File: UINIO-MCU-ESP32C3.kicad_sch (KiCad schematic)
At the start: 40 parts, among them J1 Conn_01x15_Male, J2 外接串行下载接口, J3 Conn_01x15_Male, SW1 复位按键, SW2 下载按键, U1 ME6211C33M5G-N, U2 W25Q128JVSSIQ, U3 ESP32-C3, U4 CH343P, Y1 40MHz

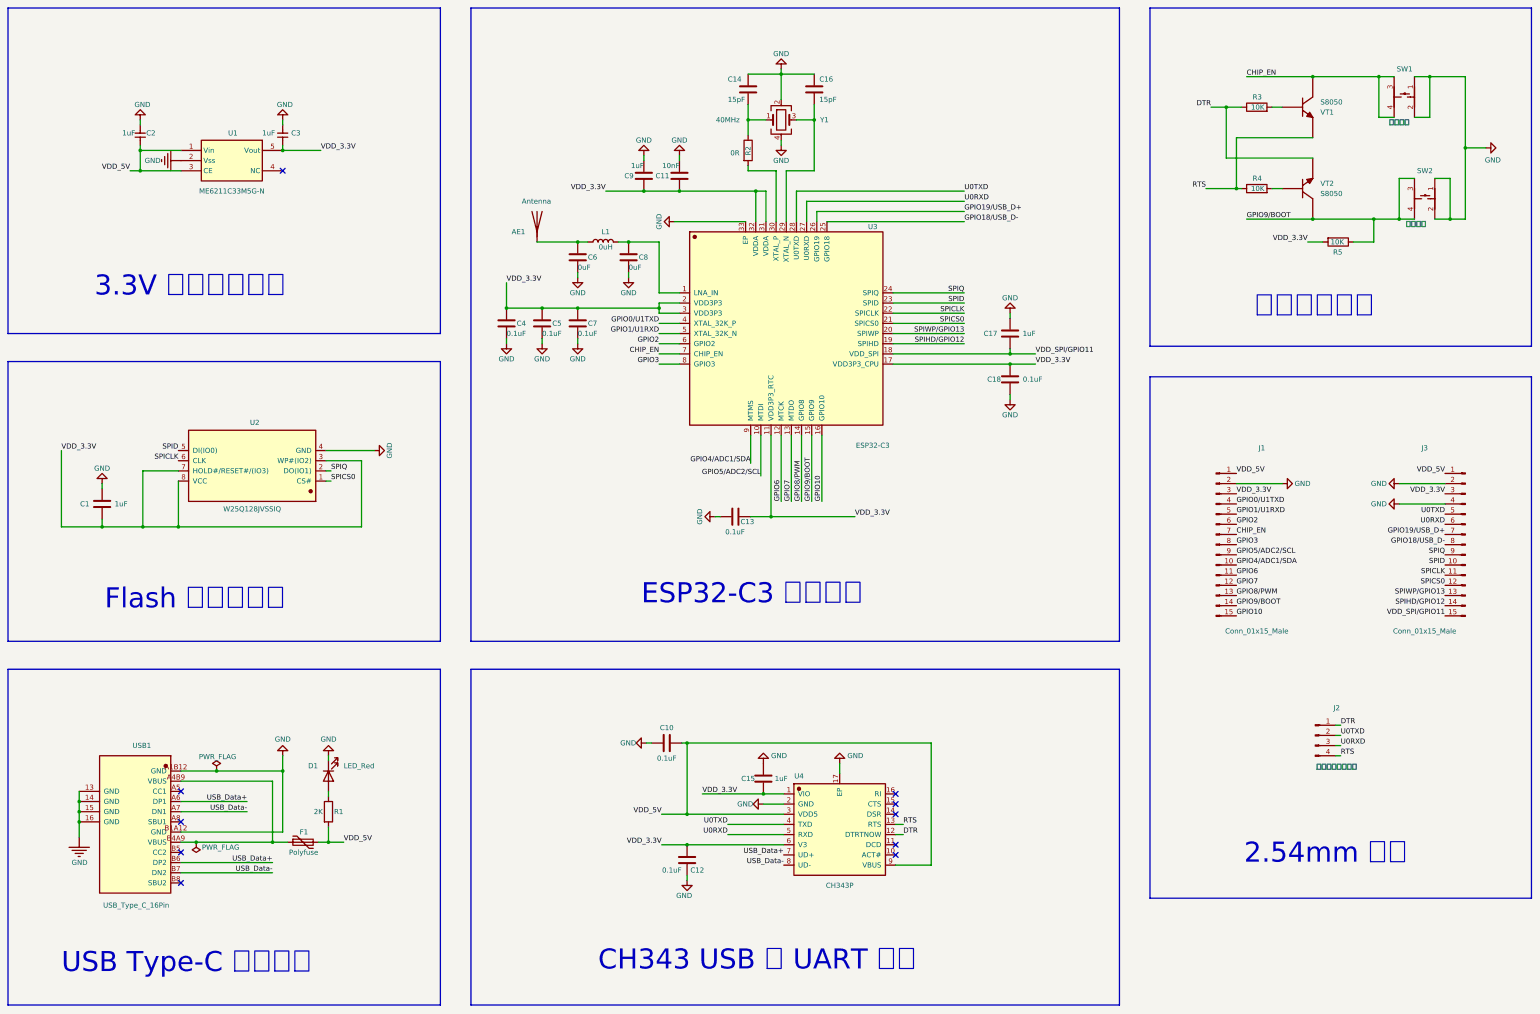
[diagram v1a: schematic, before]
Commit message: update
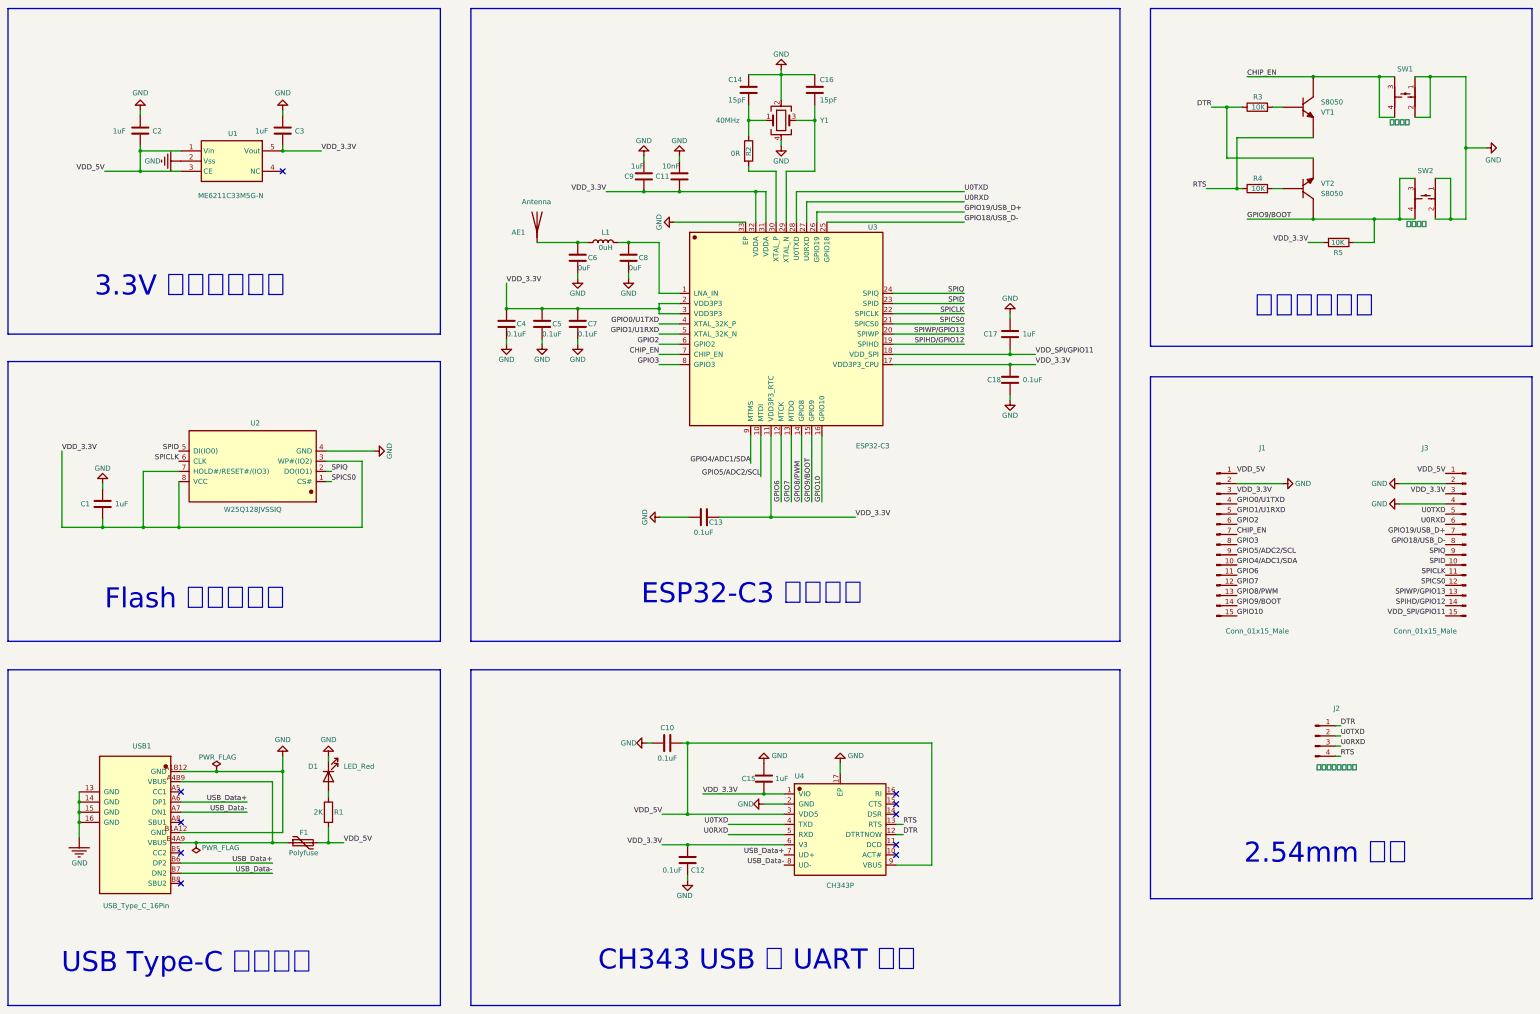
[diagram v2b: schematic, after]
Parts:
- removed C2, C3: 1uF, Capacitor_SMD:C_0402_1005Metric, symbol Uinio:CAP_0402
- added C2, C3: 1uF, Capacitor_SMD:C_0402_1005Metric, symbol Device:C
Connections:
- net GND: now also C2.1, C3.1
- net VDD_3.3V: now also C3.2
- net VDD_5V: now also C2.2
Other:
- moved on the sheet: C13
